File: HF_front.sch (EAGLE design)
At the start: 34 parts, among them U1 MC12080, U2 MAX9203, U3 HMC476MP86, U4 HMC476MP86

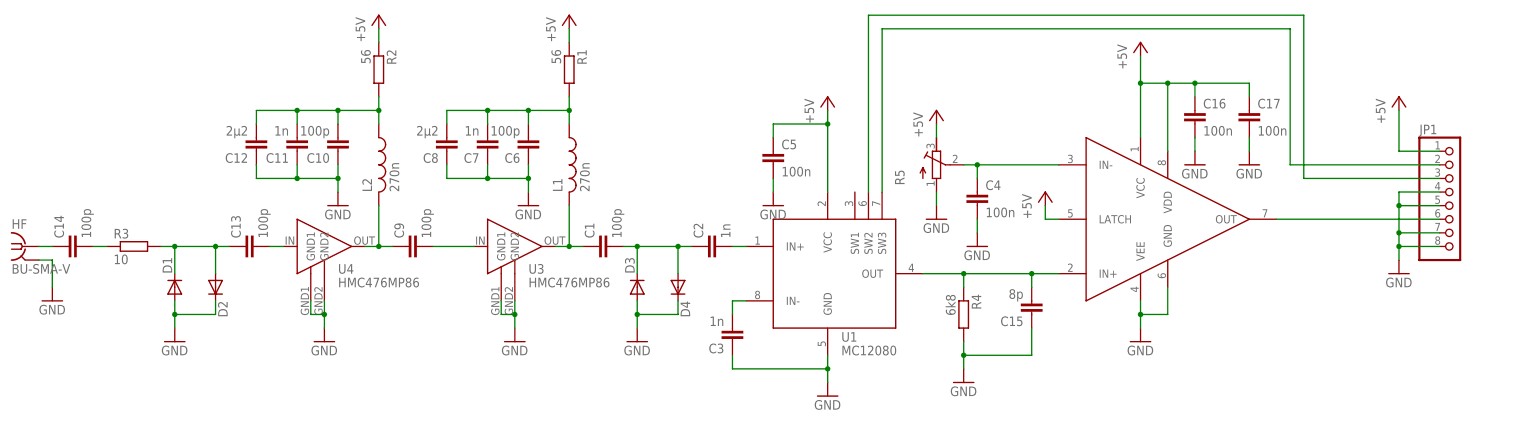
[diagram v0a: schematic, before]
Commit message: more minor pcb changes
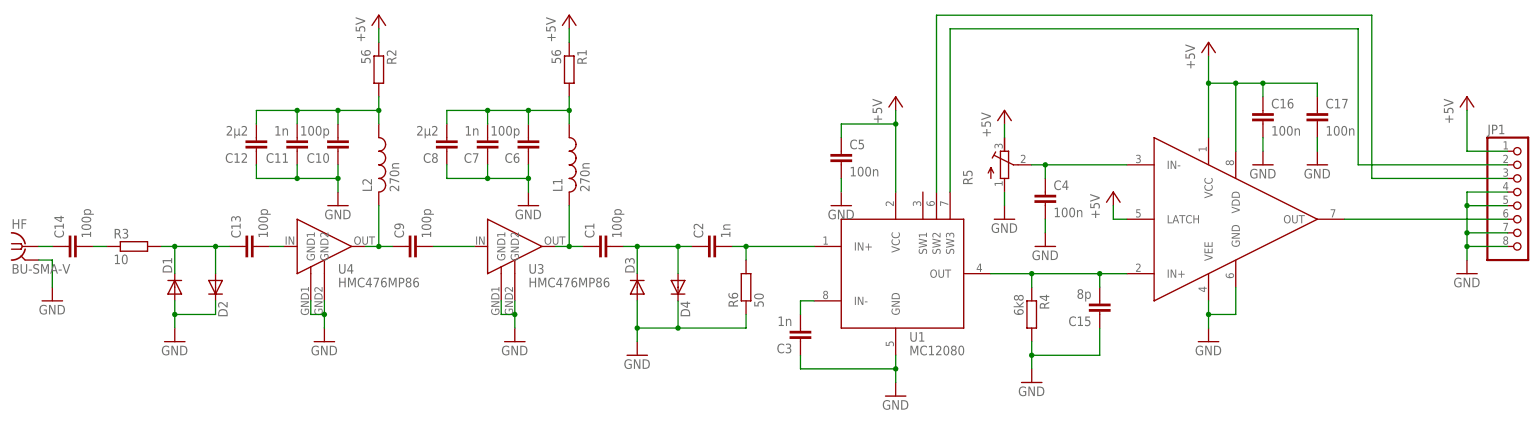
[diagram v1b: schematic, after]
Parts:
- added R6: 50, resistor:R-EU_R0603
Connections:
- net GND: now also R6.1
- net N$6: now also R6.2
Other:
- moved on the sheet: C15, C16, C17, C3, C4, C5, JP1, R4, R5, U1
